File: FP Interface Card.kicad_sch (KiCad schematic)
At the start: 23 parts, among them J1 T1M-10-F-SV-L, J4 T1M-6-F-SV-L, J5 T1M-10-F-SV-L, P1 Card Edge for HSEC8-160-01-S-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, Q17 MMBT4401-7-F, Q18 MMBT4401-7-F, Q19 IRF7404TRPBF, Q22 MMBT4401-7-F, Q23 IRF7404TRPBF, U24 RockBlock_9603

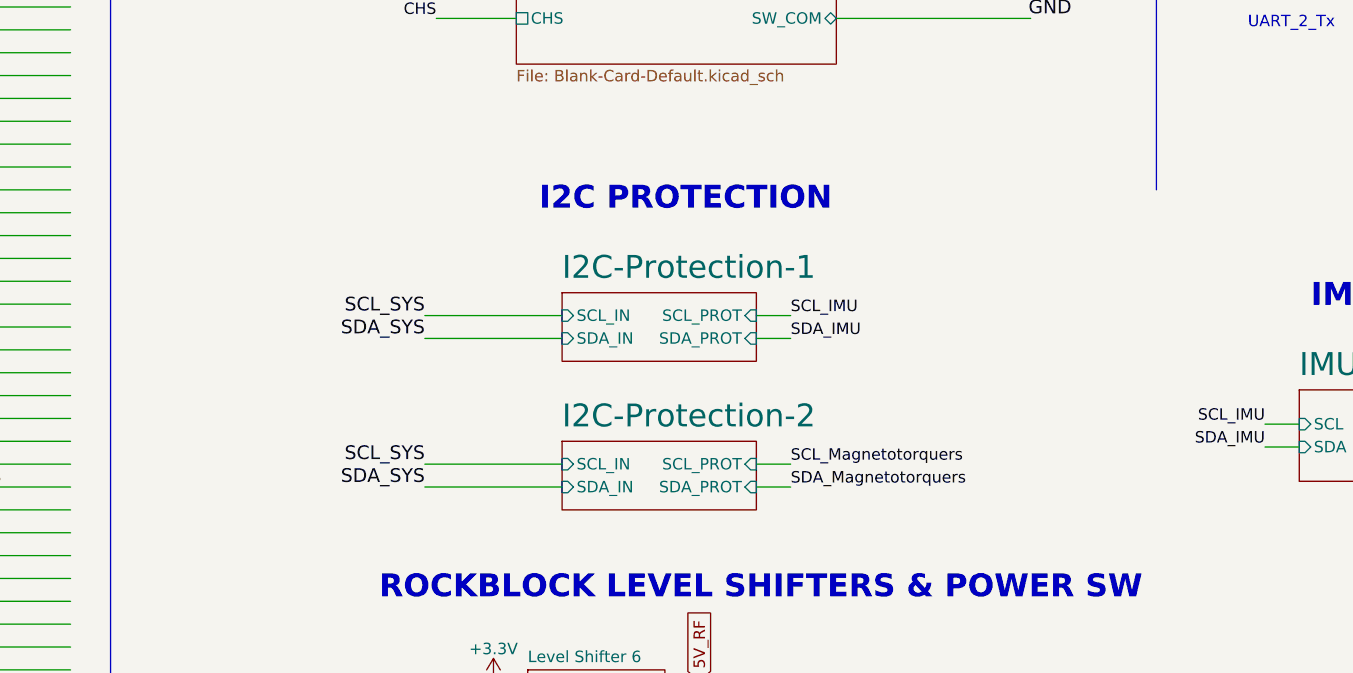
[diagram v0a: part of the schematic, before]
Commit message: updates
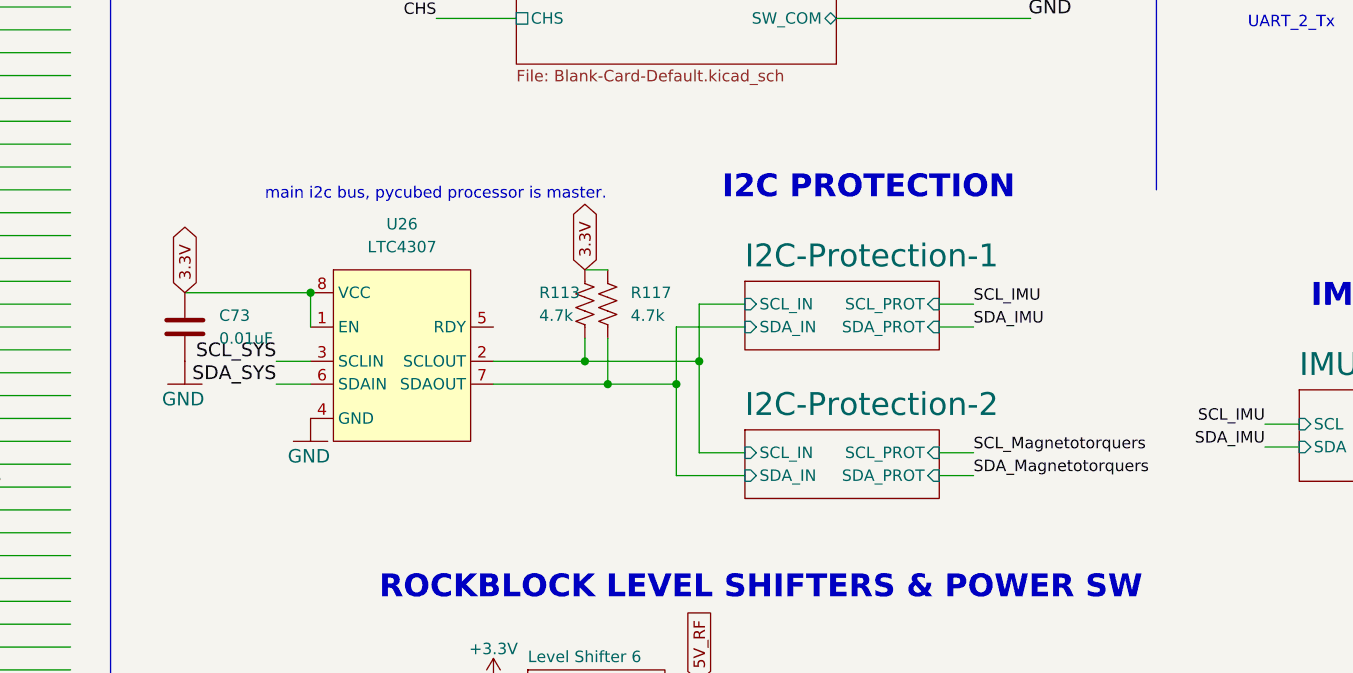
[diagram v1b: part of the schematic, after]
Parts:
- added C73: 0.01uF, Capacitor_SMD:C_0603_1608Metric, symbol Device:C
- added R113, R117: 4.7k, Resistor_SMD:R_0603_1608Metric, symbol Device:R_US
- added U26: LTC4307, Package_SO:MSOP-8_3x3mm_P0.65mm, symbol mainboard_SLI:LTC4307
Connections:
- net +3V3: now also C73.1, R113.1, R117.1, U26.1 (EN), U26.8 (VCC)
- net GND: now also C73.2, U26.4 (GND)
- net SCL_SYS: now also U26.3 (SCLIN)
- net SDA_SYS: now also U26.6 (SDAIN)
- new net I2C-Protection-1/SCL_IN: R113.2, U26.2 (SCLOUT)
- new net I2C-Protection-1/SDA_IN: R117.2, U26.7 (SDAOUT)
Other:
- note added: "main i2c bus, pycubed processor is master."
